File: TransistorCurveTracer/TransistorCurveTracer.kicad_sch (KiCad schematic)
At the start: 43 parts, among them J1 Conn_01x04_Pin, J2 Conn_01x04_Pin, J3 Conn_01x04_Pin, Q1 BC547, Q2 BC547, Q3 BC547, Q4 2N2907, Q5 2N2907, Q6 DUT, U1 NE555P, U2 MCP601-xP, U3 MCP601-xP, U4 MCP601-xP

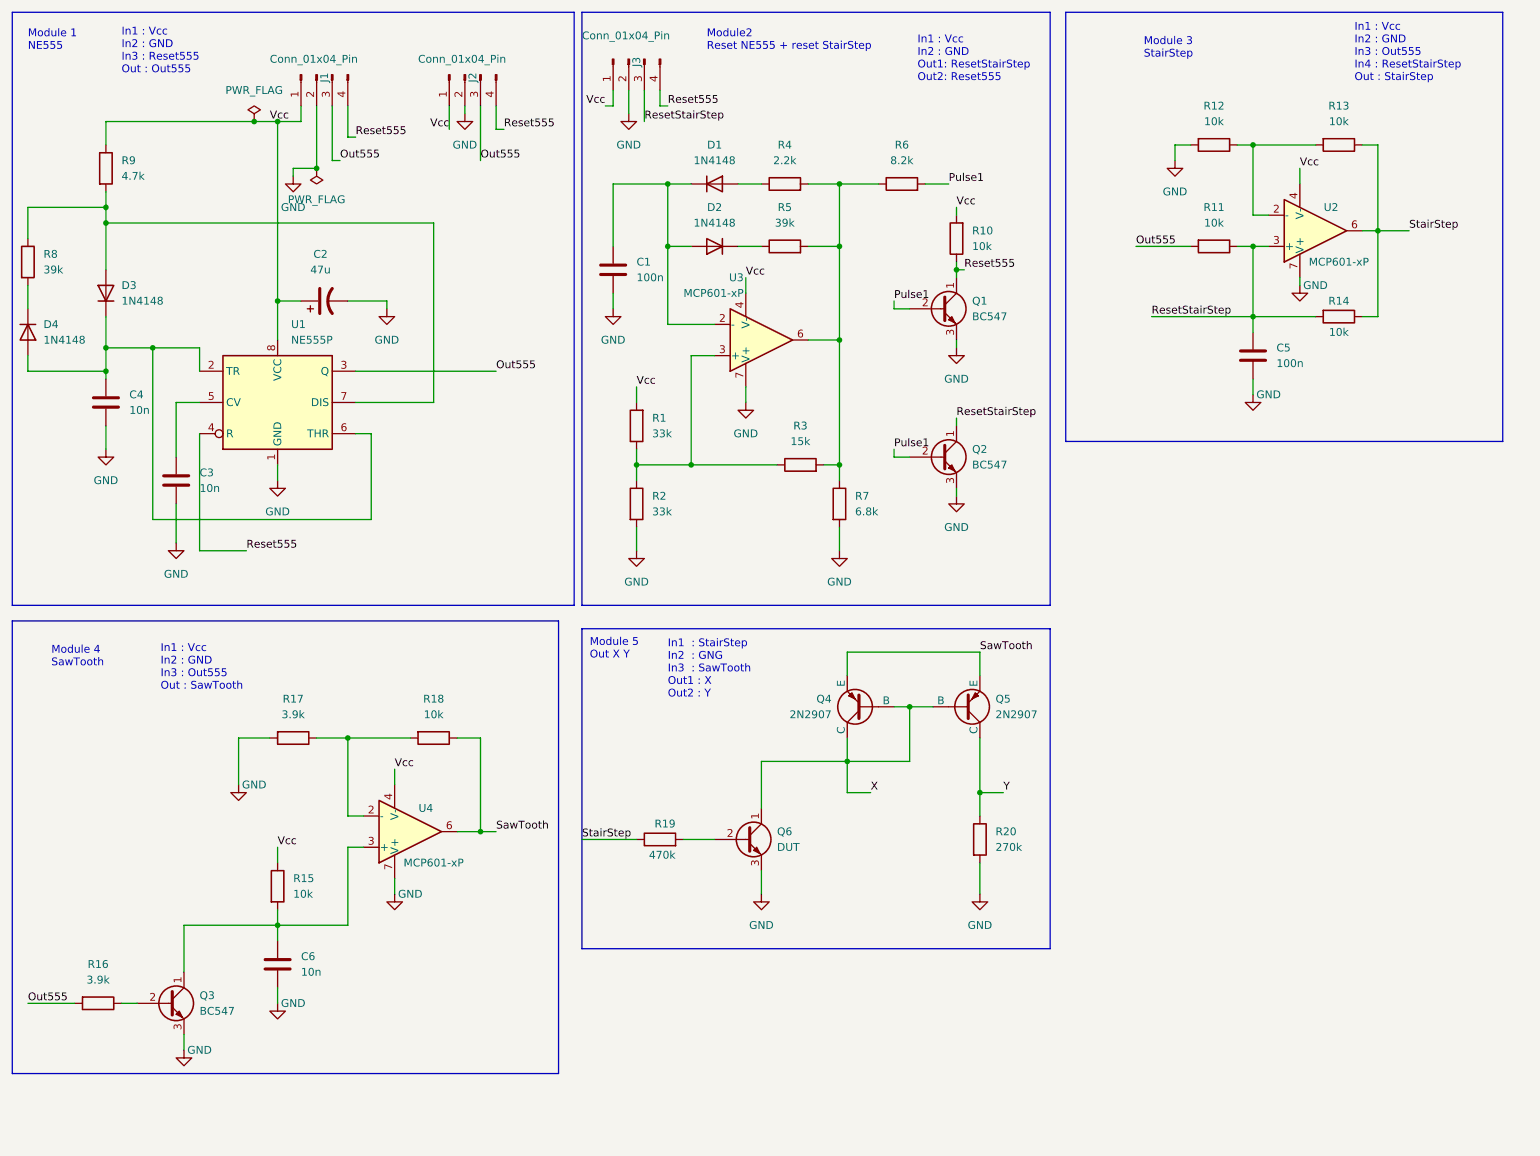
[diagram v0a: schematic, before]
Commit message: TransistorCurveTracer in progress
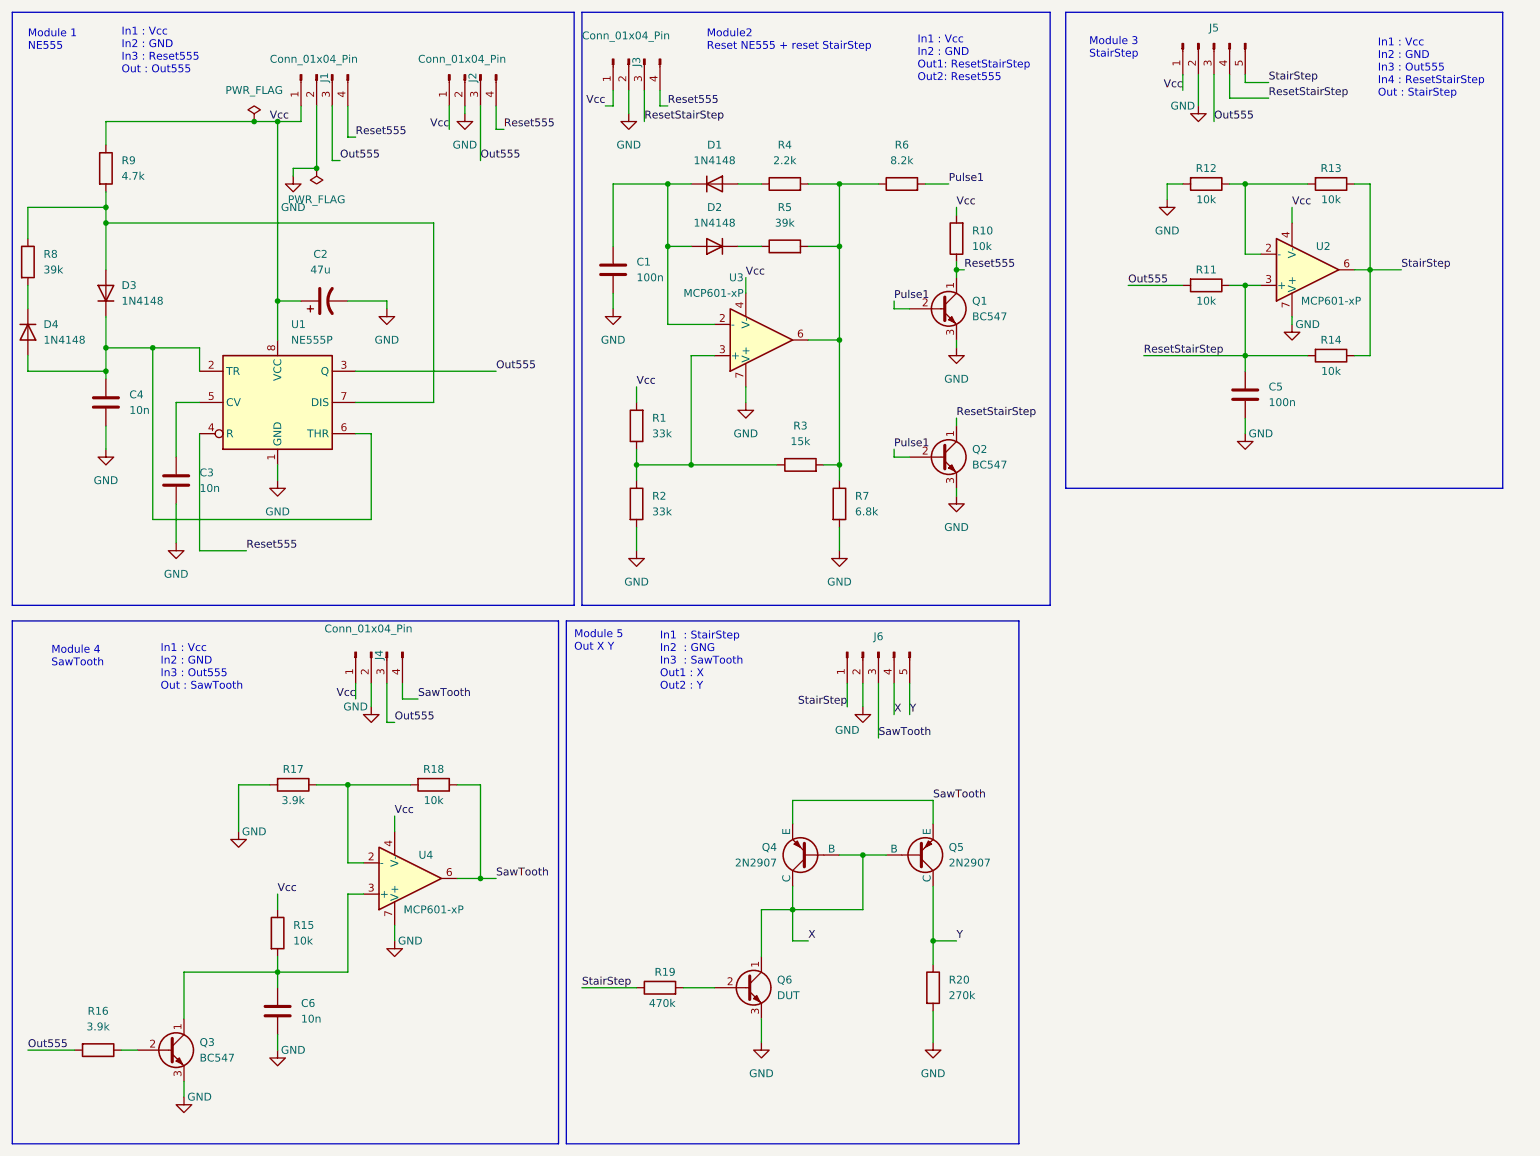
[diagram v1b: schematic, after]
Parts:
- added J4: Conn_01x04_Pin, Connector_PinHeader_2.54mm:PinHeader_1x04_P2.54mm_Vertical, symbol Connector:Conn_01x04_Pin
- added J5, J6: Conn_01x05_Pin, Connector_PinHeader_2.54mm:PinHeader_1x05_P2.54mm_Vertical, symbol Connector:Conn_01x05_Pin
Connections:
- net GND: now also J4.2 (Pin_2), J5.2 (Pin_2), J6.2 (Pin_2)
- net Out555: now also J4.3 (Pin_3), J5.3 (Pin_3)
- net ResetStairStep: now also J5.4 (Pin_4)
- net SawTooth: now also J4.4 (Pin_4), J6.3 (Pin_3)
- net StairStep: now also J5.5 (Pin_5), J6.1 (Pin_1)
- net Vcc: now also J4.1 (Pin_1), J5.1 (Pin_1)
- net X: now also J6.4 (Pin_4)
- net Y: now also J6.5 (Pin_5)
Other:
- moved on the sheet: C5, C6, Q3, Q4, Q5, Q6, R11, R12, R13, R14, R15, R16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
